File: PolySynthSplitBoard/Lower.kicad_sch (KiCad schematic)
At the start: 3 parts, among them J901 A_LOWER, J902 B_LOWER, J903 C_LOWER

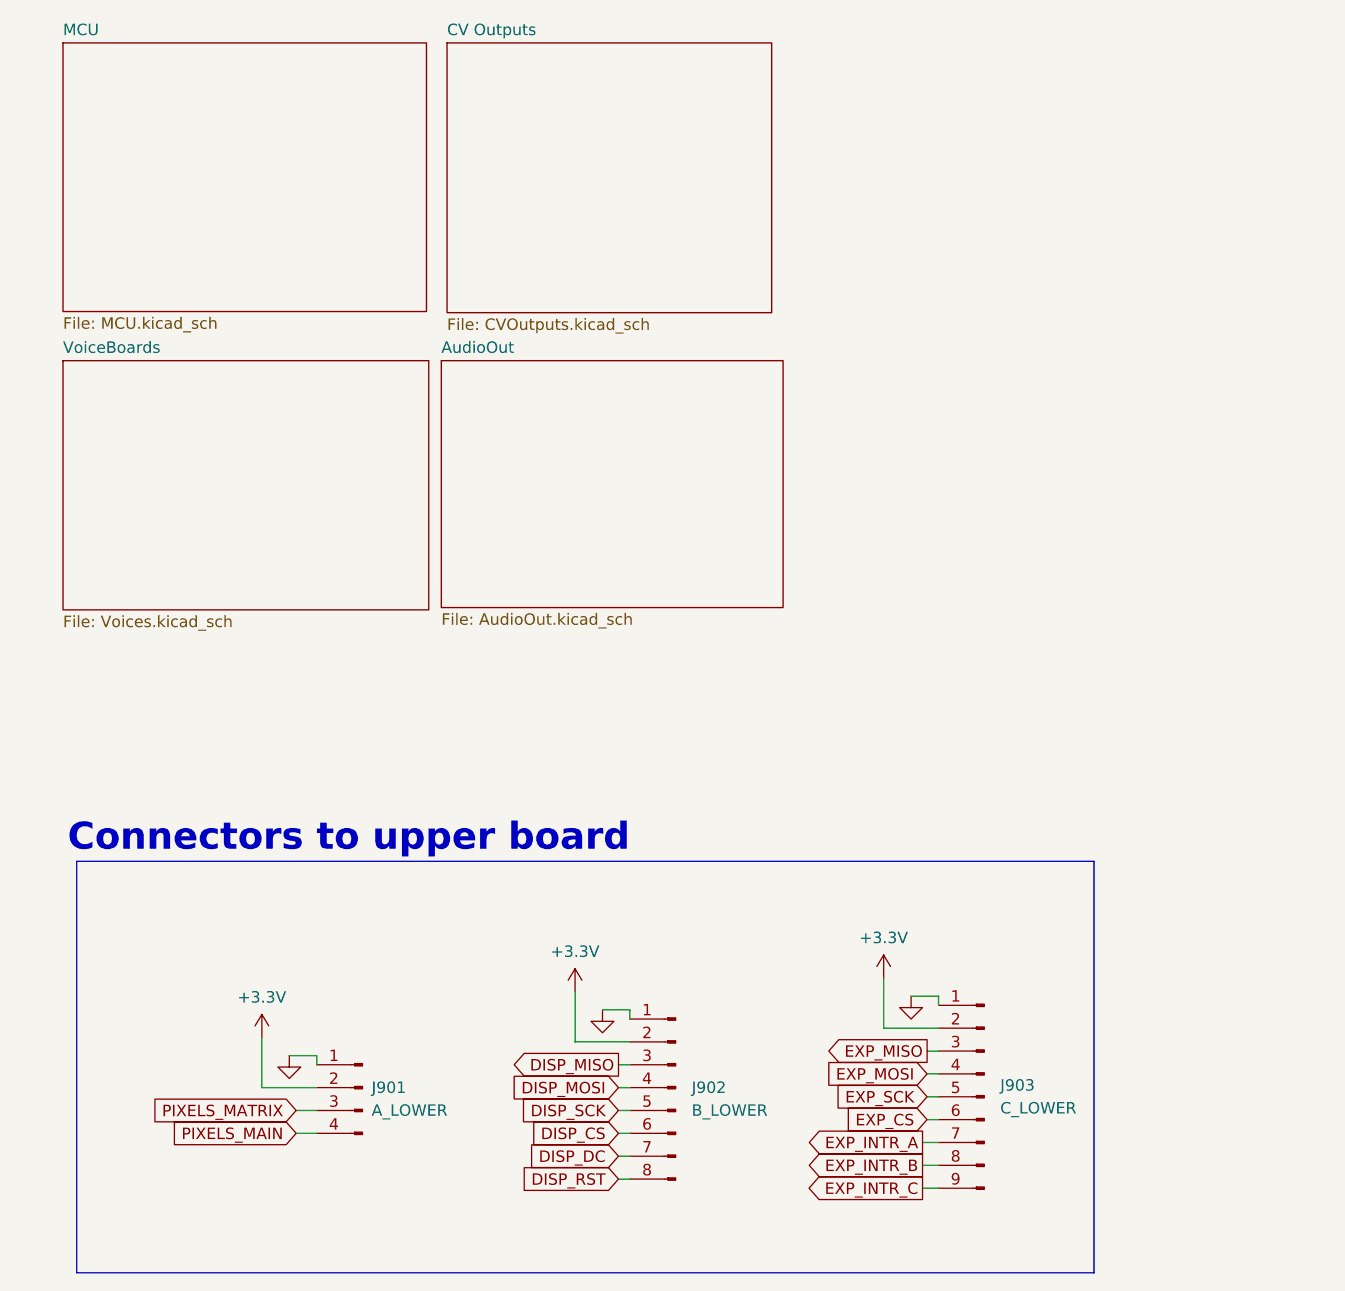
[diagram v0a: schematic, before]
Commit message: lower board
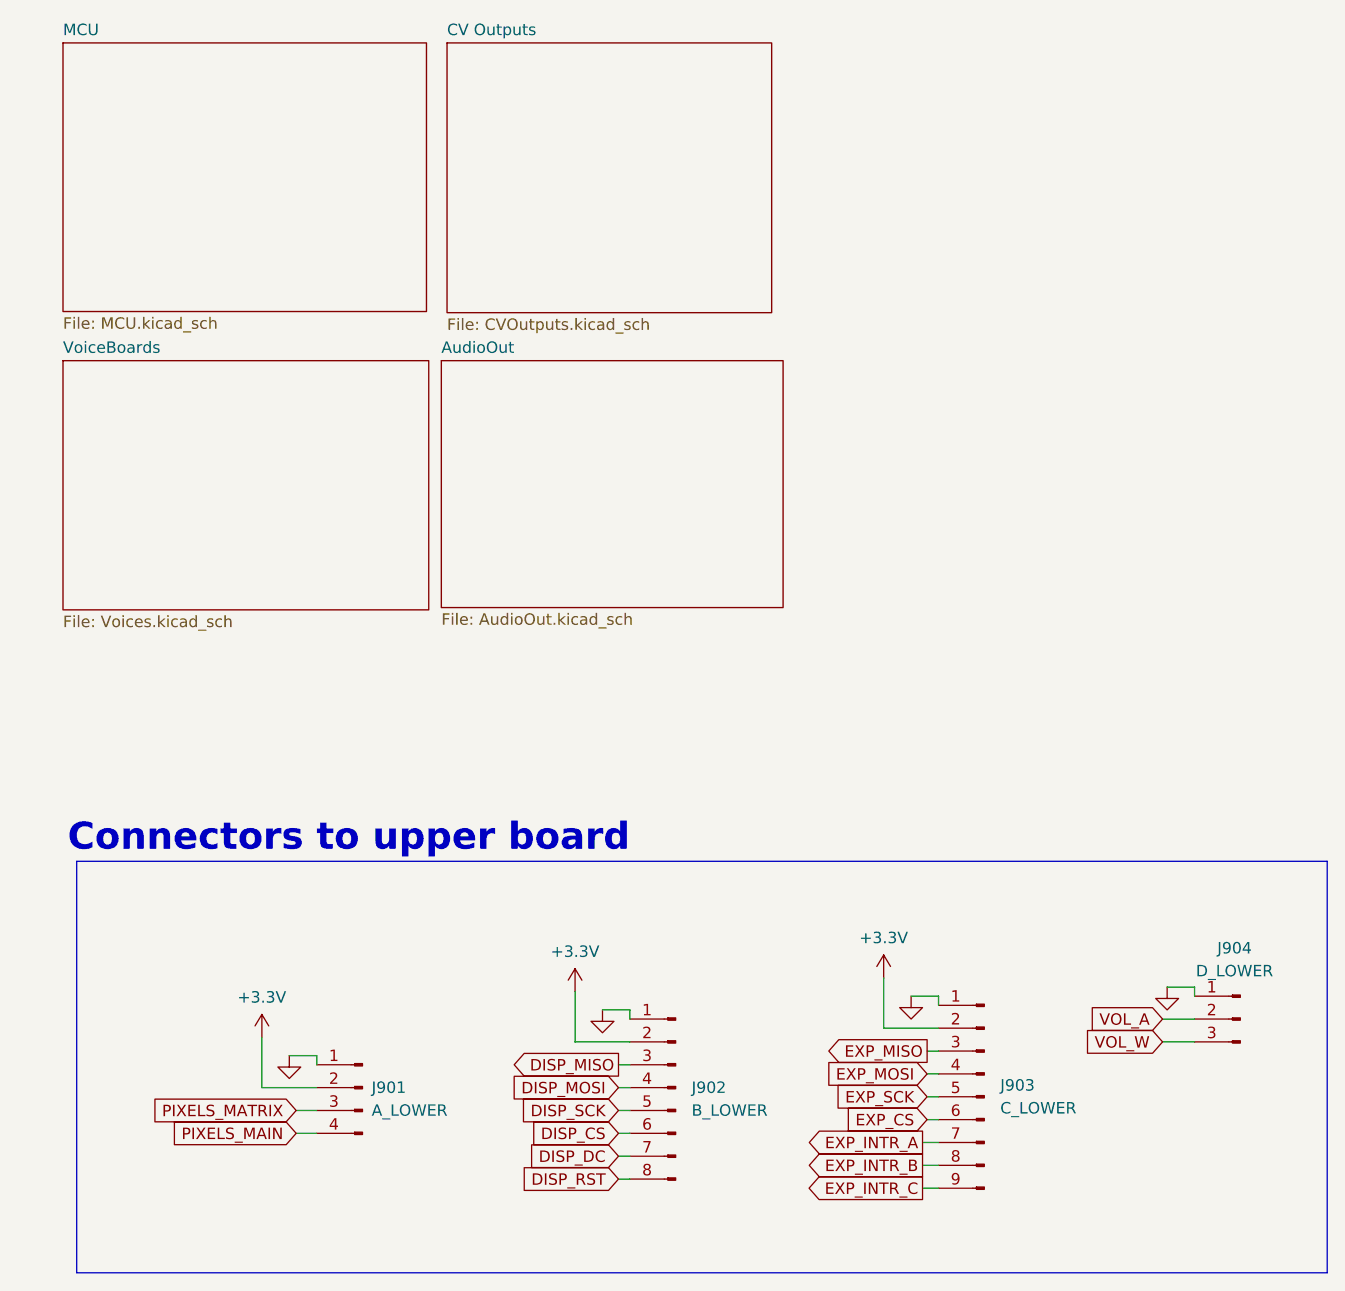
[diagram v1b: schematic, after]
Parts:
- added J904: D_LOWER, Connector_PinSocket_2.54mm:PinSocket_1x03_P2.54mm_Vertical, symbol Connector:Conn_01x03_Pin
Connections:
- net GND: now also J904.1 (Pin_1)
- new net VOL_A: J904.2 (Pin_2)
- new net VOL_W: J904.3 (Pin_3)
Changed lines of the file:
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@@
+	(wire
+		(pts
+			(xy 148.59 127.508) (xy 145.542 127.508)
+		)
+		(stroke
+			(width 0)
+			(type default)
+		)
+	)
 	(wire
 		(pts
@@
 	(wire
 		(pts
+			(xy 148.59 128.524) (xy 148.59 127.508)
+		)
+		(stroke
+			(width 0)
+			(type default)
+		)
+	)
+	(wire
+		(pts
+			(xy 145.034 131.064) (xy 148.59 131.064)
+		)
+		(stroke
+			(width 0)
+			(type default)
+		)
+	)
+	(wire
+		(pts
 			(xy 85.852 131.064) (xy 85.852 130.048)
 		)
@@
 		(pts
 			(xy 84.582 146.304) (xy 85.852 146.304)
+		)
+		(stroke
+			(width 0)
+			(type default)
+		)
+	)
+	(wire
+		(pts
+			(xy 145.034 133.604) (xy 148.59 133.604)
 		)
 		(stroke
@@
 	(rectangle
 		(start 24.384 113.538)
-		(end 137.414 159.258)
+		(end 163.322 159.258)
 		(stroke
 			(width 0)
@@
 		)
 	)
+	(global_label "VOL_A"
+		(shape input)
+		(at 145.034 131.064 180)
+		(fields_autoplaced yes)
+		(effects
+			(font
+				(size 1.27 1.27)
+			)
+			(justify right)
+		)
+		(property "Intersheetrefs" "${INTERSHEET_REFS}"
+			(at 136.5454 131.064 0)
+			(effects
+				(font
+					(size 1.27 1.27)
+				)
+				(justify right)
+				(hide yes)
+			)
+		)
+	)
 	(global_label "EXP_MOSI"
 		(shape input)
@@
 		(property "Intersheetrefs" "${INTERSHEET_REFS}"
 			(at 71.4368 146.304 0)
+			(effects
+				(font
+					(size 1.27 1.27)
+				)
+				(justify right)
+				(hide yes)
+			)
+		)
+	)
+	(global_label "VOL_W"
+		(shape input)
+		(at 145.034 133.604 180)
+		(fields_autoplaced yes)
+		(effects
+			(font
+				(size 1.27 1.27)
+			)
+			(justify right)
+		)
+		(property "Intersheetrefs" "${INTERSHEET_REFS}"
+			(at 136.1826 133.604 0)
 			(effects
 				(font
@@
 				(path "/22649217-9810-470f-bc7b-6f743ad2b90e/3d9ecb3b-9556-42d6-955a-a32d9efd5d3a"
 					(reference "#PWR0902")
+					(unit 1)
+				)
+			)
+		)
+	)
+	(symbol
+		(lib_id "Connector:Conn_01x03_Pin")
+		(at 153.67 131.064 0)
+		(mirror y)
+		(unit 1)
+		(exclude_from_sim no)
+		(in_bom yes)
+		(on_board yes)
+		(dnp no)
+		(property "Reference" "J904"
+			(at 153.035 123.19 0)
+			(effects
+				(font
+					(size 1.27 1.27)
+				)
+			)
+		)
+		(property "Value" "D_LOWER"
+			(at 153.035 125.73 0)
+			(effects
+				(font
+					(size 1.27 1.27)
+				)
+			)
+		)
+		(property "Footprint" "Connector_PinSocket_2.54mm:PinSocket_1x03_P2.54mm_Vertical"
+			(at 153.67 131.064 0)
+			(effects
+				(font
+					(size 1.27 1.27)
+				)
+				(hide yes)
+			)
+		)
+		(property "Datasheet" "~"
+			(at 153.67 131.064 0)
+			(effects
+				(font
+					(size 1.27 1.27)
+				)
+				(hide yes)
+			)
+		)
+		(property "Description" "Generic connector, single row, 01x03, script generated"
+			(at 153.67 131.064 0)
+			(effects
+				(font
+					(size 1.27 1.27)
+				)
+				(hide yes)
+			)
+		)
+		(pin "2"
+		)
+		(pin "1"
+		)
+		(pin "3"
+		)
+		(instances
+			(project ""
+				(path "/22649217-9810-470f-bc7b-6f743ad2b90e/3d9ecb3b-9556-42d6-955a-a32d9efd5d3a"
+					(reference "J904")
 					(unit 1)
 				)
@@
 					(unit 1)
 				)
+			)
+		)
+	)
+	(symbol
+		(lib_id "power:GND")
+		(at 145.542 127.508 0)
+		(unit 1)
+		(exclude_from_sim no)
+		(in_bom yes)
+		(on_board yes)
+		(dnp no)
+		(fields_autoplaced yes)
+		(property "Reference" "#PWR0907"
+			(at 145.542 133.858 0)
+			(effects
+				(font
+					(size 1.27 1.27)
+				)
+				(hide yes)
+			)
+		)
+		(property "Value" "GND"
+			(at 145.542 131.318 0)
+			(effects
+				(font
+					(size 1.27 1.27)
+				)
+				(hide yes)
+			)
+		)
+		(property "Footprint" ""
+			(at 145.542 127.508 0)
+			(effects
+				(font
+					(size 1.27 1.27)
+				)
+				(hide yes)
+			)
+		)
+		(property "Datasheet" ""
+			(at 145.542 127.508 0)
+			(effects
+				(font
+					(size 1.27 1.27)
+				)
+				(hide yes)
+			)
+		)
+		(property "Description" ""
+			(at 145.542 127.508 0)
+			(effects
+				(font
+					(size 1.27 1.27)
+				)
+				(hide yes)
+			)
+		)
+		(pin "1"
+		)
+		(instances
+			(project "PolySynthSplitBoard"
+				(path "/22649217-9810-470f-bc7b-6f743ad2b90e/3d9ecb3b-9556-42d6-955a-a32d9efd5d3a"
+					(reference "#PWR0907")
+					(unit 1)
+				)
